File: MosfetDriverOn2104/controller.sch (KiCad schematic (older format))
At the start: 22 parts, among them SW1 SW_Push, SW2 SW_Push, SW3 SW_DIP_x04, SW4 SW_Push, U1 ATmega328P-AU-MCU_Microchip_A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

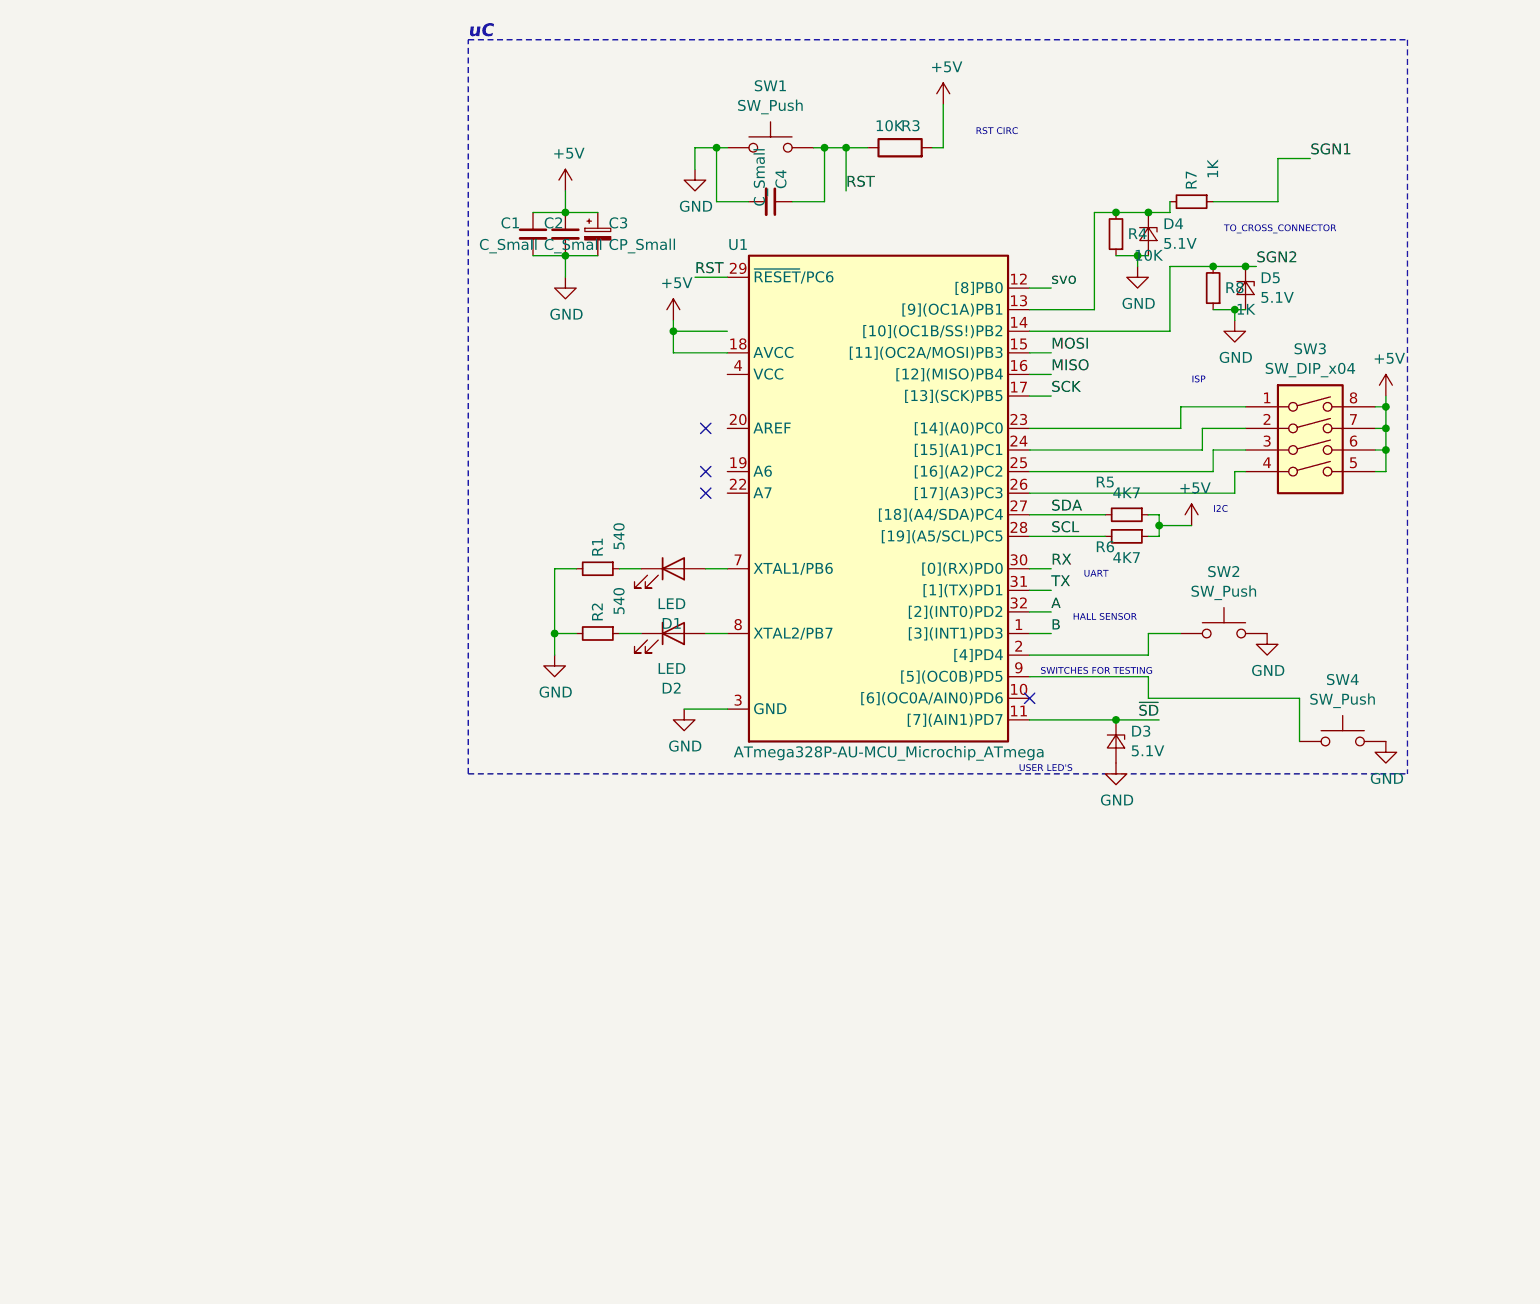
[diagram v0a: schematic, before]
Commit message: Sorted PCB
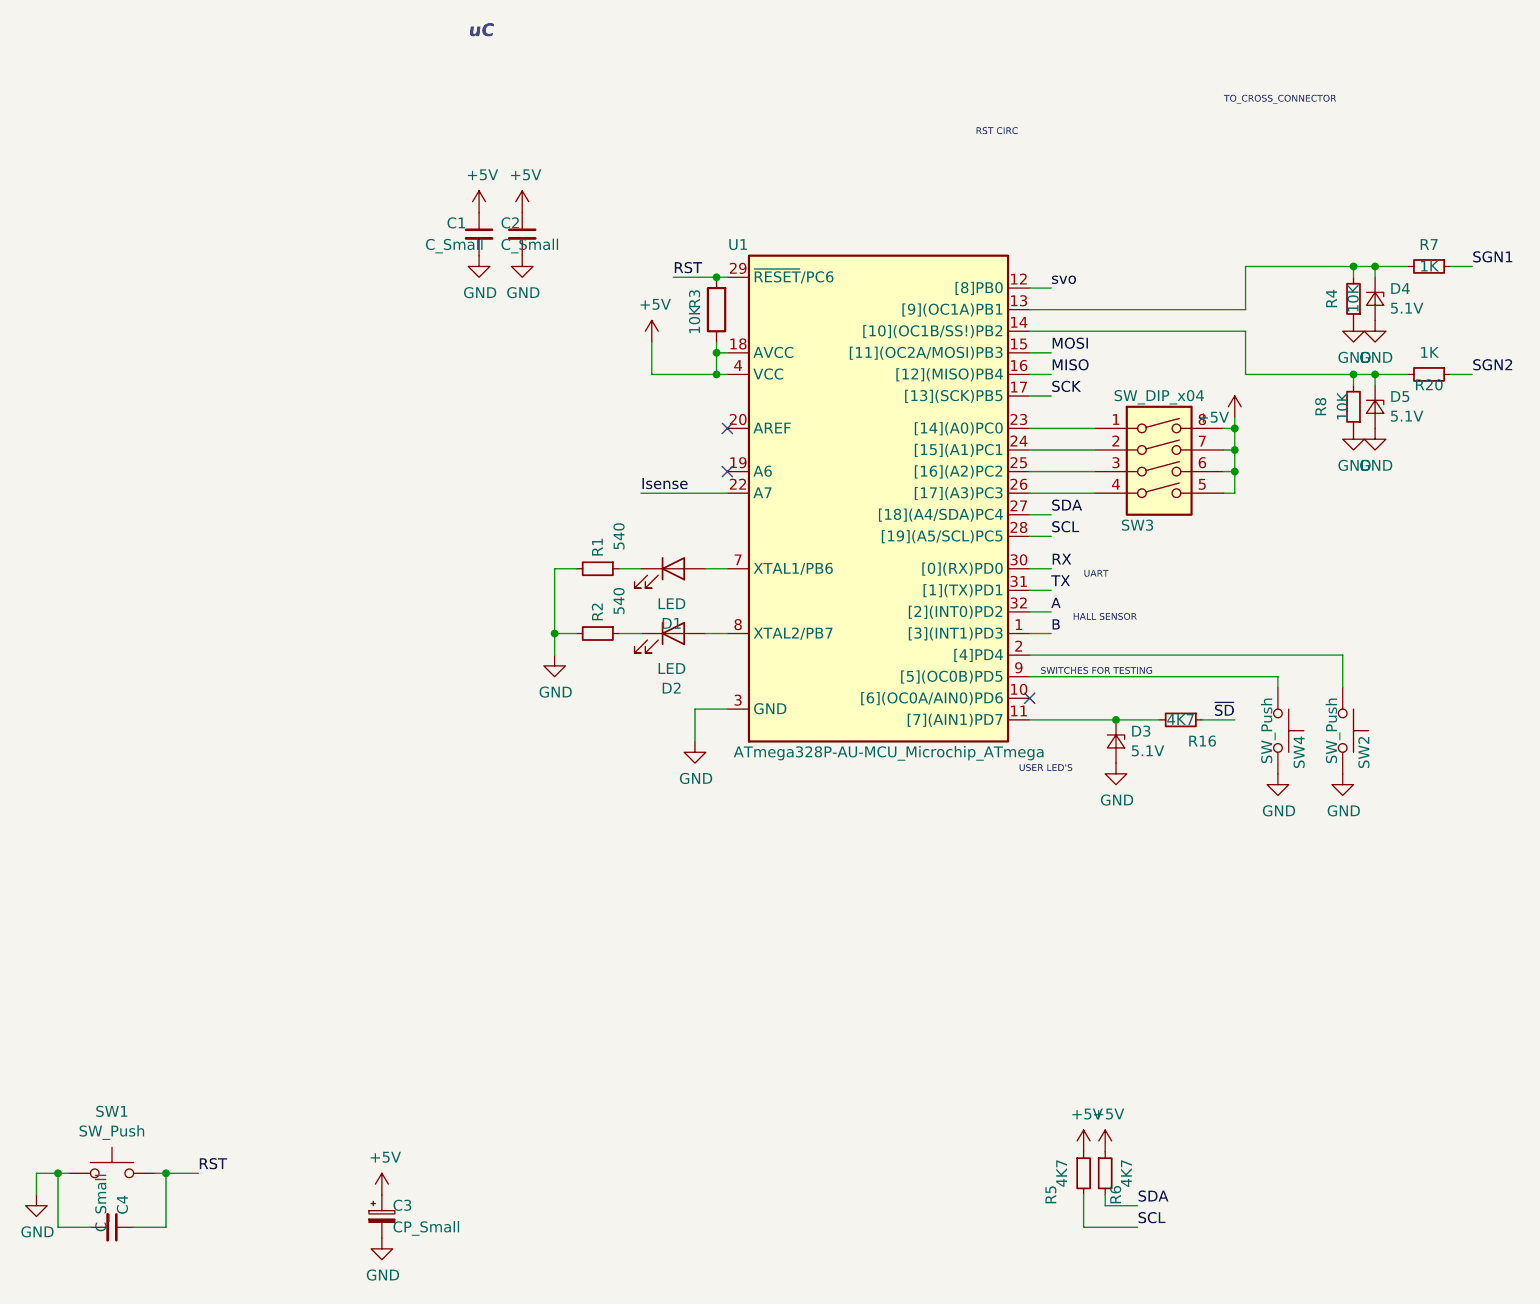
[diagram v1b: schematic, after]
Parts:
- added R16: 4K7, Resistor_SMD:R_0805_2012Metric, symbol Device:R_Small
- added R20: 1K, Resistor_SMD:R_0805_2012Metric, symbol Device:R_Small
- R8: value 1K -> 10K
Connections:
- net +5V: now also R3.1, U1.4 (VCC), U1.6 (VCC); no longer R3.2
- net RST: now also R3.2; no longer R3.1
- net SCL: now also R5.2; no longer R6.2
- net SDA: now also R6.2; no longer R5.2
- net SGN2: now also R20.1; no longer D5.1 (K), R8.2, U1.14 ([10](OC1B/SS!)PB2)
- net ~SD: now also R16.1; no longer D3.1 (K), U1.11 ([7](AIN1)PD7)
- net Isense: now reaches U1.22 (A7)
- new net: D3.1 (K), R16.2, U1.11 ([7](AIN1)PD7)
- new net: D5.1 (K), R20.2, R8.2, U1.14 ([10](OC1B/SS!)PB2)
- no-connect marks 4 -> 3
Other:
- note removed: "I2C\n"
- note removed: "ISP"
- moved on the sheet: C1, C2, C3, C4, D4, D5, R3, R4, R5, R6, R7, R8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
